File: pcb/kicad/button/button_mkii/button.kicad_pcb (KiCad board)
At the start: 2 copper layers, 168 parts, among them J1 SWD with less, U1 STBlueNRG-1, Y1 Xtal 32.768kHz, Y2 XTAL 16MHz

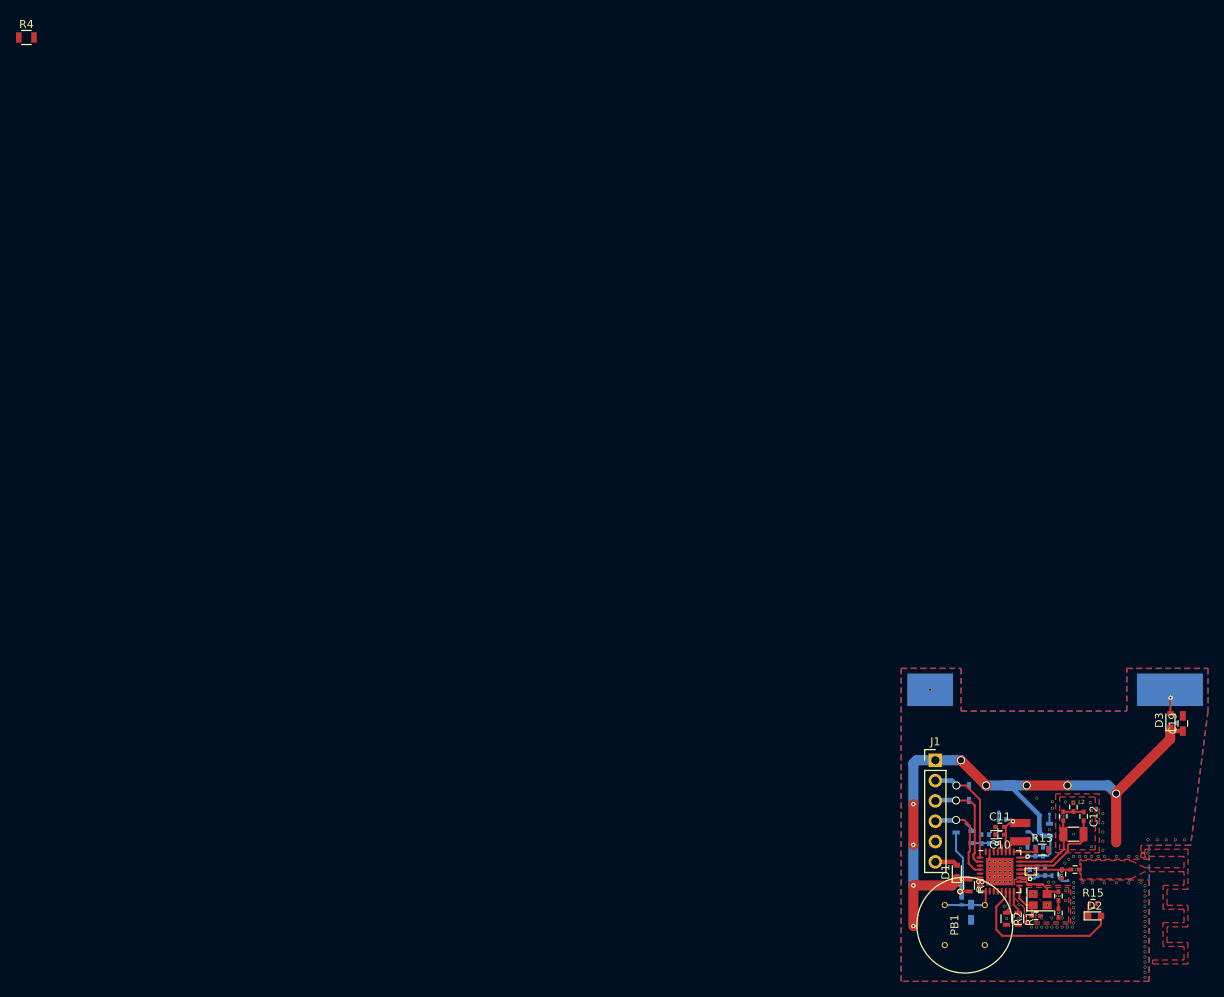
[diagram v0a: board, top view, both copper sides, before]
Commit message: updated design, layout, and appnotes; rev3
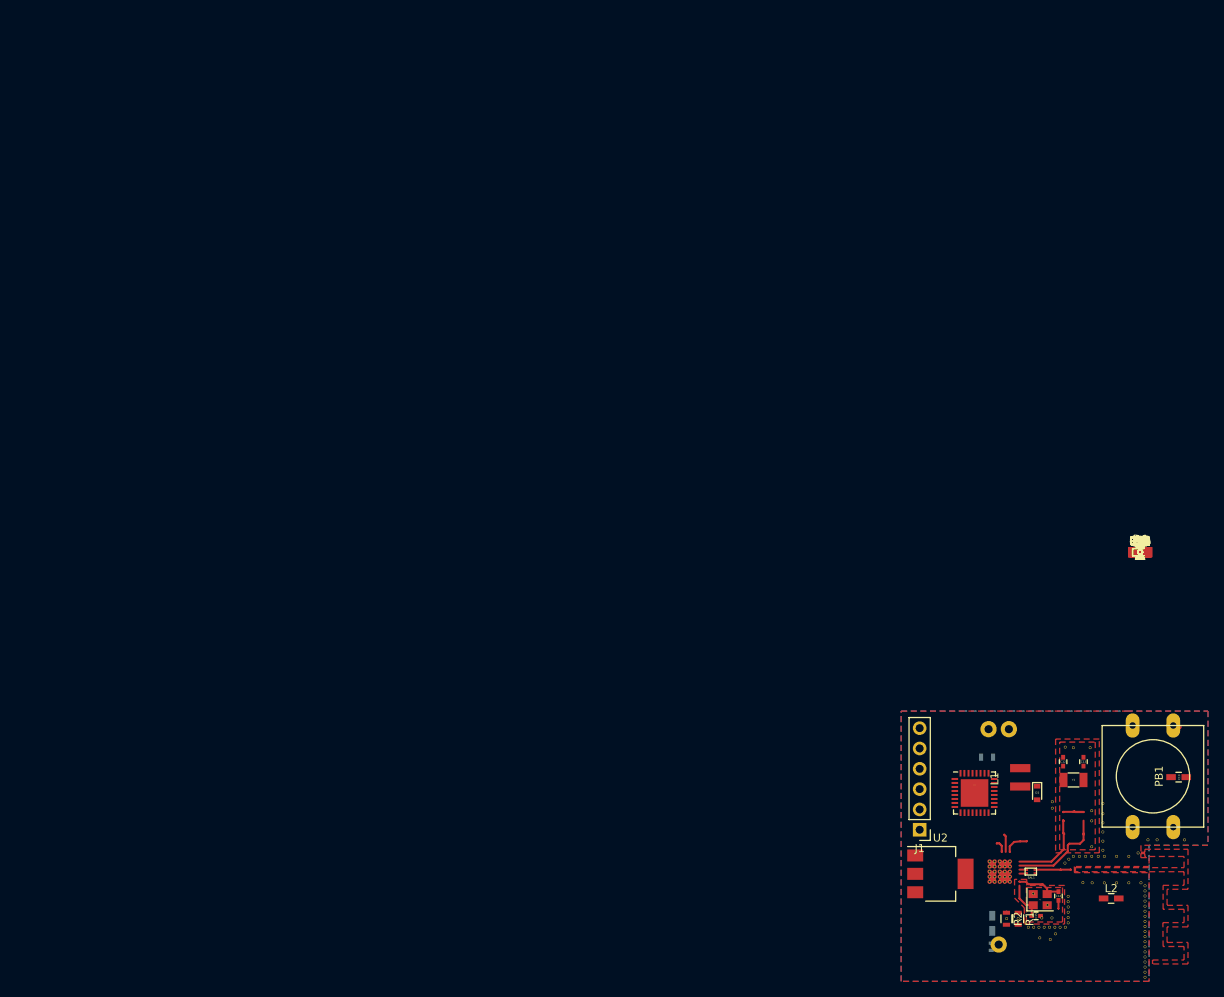
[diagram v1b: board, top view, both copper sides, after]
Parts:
- removed L3: RFC, Miscellaneous:L_0402
- removed the REF** at (127.9, 99.0)
- removed the REF** at (122.2, 108.6)
- removed the REF** at (130.9, 105.6)
- removed the REF** at (124.2, 101.3)
- removed the REF** at (130.9, 106.2)
- removed the REF** at (124.1, 108.4)
- removed the REF** at (113.0, 81.5)
- removed the REF** at (140.2, 101.9)
- removed the REF** at (130.9, 106.9)
- removed the REF** at (143.6, 100.3)
- removed the REF** at (142.5, 100.3)
- removed the REF** at (127.8, 105.6)
- removed the REF** at (128.4, 105.6)
- removed the REF** at (130.9, 107.5)
- added C20, C21: 1uF, Capacitors_SMD:C_0402, F.Cu at (139.2, 64.3)
- added C22: 1uF, Capacitors_SMD:C_0805, F.Cu at (139.2, 64.3)
- added C23: 0.1uF, Capacitors_SMD:C_0603, F.Cu at (139.2, 64.3)
- added C24: 0.01uF, Capacitors_SMD:C_0402, F.Cu at (139.2, 64.3)
- added R16: 1k, Resistors_SMD:R_0402, F.Cu at (139.2, 64.3)
- added R17: 100k, Resistors_SMD:R_0402, F.Cu at (139.2, 64.3)
- added TP7: Xtal32MHz, Miscellaneous:Measurement_Point_Round-SMD-tiniest, F.Cu at (139.2, 64.3)
- added TP8: Xtal32kHz, Miscellaneous:Measurement_Point_Round-SMD-tiniest, F.Cu at (139.2, 64.3)
- added U2: TLV1117LV-3V, TO_SOT_Packages_SMD:SOT-223, F.Cu at (114.2, 104.5)
- BT1: footprint Batteries:SMD_CoinCell -> Batteries:CoinCell_holder_1060x630
- C1: value 100pF -> 1uF; footprint Capacitors_SMD:C_0402 -> Capacitors_SMD:C_0805; moved to F.Cu
- C14: value 22pF -> 27pF
- C15: value 18pF -> 33pF
- C18: value CP -> 1uF
- C2: footprint Capacitors_SMD:C_0402 -> Capacitors_SMD:C_0603; moved to F.Cu
- C3: value 2.2pF -> 0.01uF; moved to F.Cu
- C4: value 1000pF -> 0.01uF; footprint Capacitors_SMD:C_0402 -> Capacitors_SMD:C_0805; moved to F.Cu
- C5: value 2.2uF -> 1000pF; footprint Capacitors_SMD:C_0402 -> Capacitors_SMD:C_0603; moved to F.Cu
- C6, R10, R11, R12, R3, R7, R9, TP1, TP3, TP4, TP5, TP6: moved to F.Cu
- C7: value 10pF -> 0.01uF; footprint Capacitors_SMD:C_0402 -> Capacitors_SMD:C_0805; moved to F.Cu
- C8: value 1uF -> 1000pF; footprint Capacitors_SMD:C_0402 -> Capacitors_SMD:C_0603; moved to F.Cu
- C9: value 1000pF -> 10pF; moved to F.Cu
- D1: value Power thru SWD -> LED (Green-1); footprint Diodes_SMD:D_0603 -> LEDs:LED_0402
- D2: value LED -> LED (Green-2); footprint LEDs:LED_0603 -> LEDs:LED_0402
- L2: value RFC -> L; footprint Miscellaneous:L_0402 -> Capacitors_SMD:C_0603_HandSoldering
- PB1: value pb_basic -> pb_v2; footprint Miscellaneous:pb_basic -> Buttons_Switches_THT:SW_PUSH-12mm
- R14: value 10k -> 1k
- R6: value 100k -> 1k; footprint Resistors_SMD:R_0603 -> Resistors_SMD:R_0402; moved to F.Cu
- U1: footprint uCs:STBNRG1 -> STBNRG1
- Y2: value XTAL 16MHz -> XTAL 32MHz
- moved R4 153.4 mm to (139.2, 64.3)
- moved TP2 48.0 mm to (139.2, 64.3)
- moved R8 46.8 mm to (139.2, 64.3), turned to 0 degrees
- moved D1 46.1 mm to (139.2, 64.3), turned to 0 degrees
- moved D2 45.8 mm to (139.2, 64.3)
- moved R15 44.3 mm to (139.2, 64.3)
- moved C5 42.5 mm to (139.2, 64.3), turned to 0 degrees
- moved TP3 42.0 mm to (139.2, 64.3)
- moved C6 41.9 mm to (139.2, 64.3), turned to 0 degrees
- moved R9 41.8 mm to (139.2, 64.3)
- moved C4 41.6 mm to (139.2, 64.3), turned to 0 degrees
- moved C16 41.4 mm to (139.2, 64.3), turned to 0 degrees
- moved R7 41.3 mm to (139.2, 64.3), turned to 0 degrees
- moved R6 41.3 mm to (139.2, 64.3), turned to 0 degrees
- moved C3 41.0 mm to (139.2, 64.3), turned to 0 degrees
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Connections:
- net RF0 renamed /RF0
- net RF1 renamed /RF1
- BT1 pad 2: GND -> Net-(BT1-Pad1)
- C12 pad 1: Net-(C12-Pad1) -> GND
- C13 pad 1: Net-(C12-Pad1) -> GND
- C14 pad 1: Net-(C14-Pad1) -> GND
- C17 pad 2: Net-(BAL1-Pad3) -> GND
- C18 pad 1: DIO3 -> +3V3
- C18 pad 2: GND -> /DIO12_BUTTON
- C19 pad 1: +3V3 -> Net-(BT1-Pad1)
- C4 pad 1: GND -> +3V3
- C4 pad 2: +3V3 -> GND
- C5 pad 1: GND -> +3V3
- C5 pad 2: +3V3 -> GND
- C6 pad 1: GND -> +3V3
- C6 pad 2: +3V3 -> GND
- D1 pad 1: +3V3 -> GND
- D2 pad 2: ANATEST1 -> /DIO3_LED
- J1 pad 1: +3V3 -> Net-(C20-Pad2)
- J1 pad 2: DIO10 -> DIO7
- J1 pad 4: DIO7 -> DIO10
- J1 pad 6: Net-(D1-Pad2) -> +3V3
- L2 pad 1: Net-(C12-Pad1) -> Net-(BAL1-Pad3)
- PB1 pad 1: DIO3 -> +3V3
- PB1 pad 2: GND -> /DIO12_BUTTON
- R13 pad 1: RESET -> GND
- R13 pad 2: GND -> Net-(R13-Pad2)
- R14 pad 1: +3V3 -> /DIO12_BUTTON
- R14 pad 2: DIO3 -> Net-(D1-Pad2)
- R4 pad 1: DIO10 -> +3V3
- R4 pad 2: +3V3 -> DIO7
- R6 pad 1: DIO7 -> Net-(C14-Pad2)
- R6 pad 2: +3V3 -> Net-(R6-Pad2)
- R7 pad 1: Net-(C1-Pad1) -> Net-(R7-Pad1)
- R7 pad 2: Net-(R7-Pad2) -> Net-(C1-Pad1)
- R8 pad 1: +3V3 -> Net-(R8-Pad1)
- R8 pad 2: Net-(R8-Pad2) -> +3V3
- TP1 pad 1: Net-(R7-Pad2) -> Net-(R7-Pad1)
- TP2 pad 1: Net-(R8-Pad2) -> Net-(R8-Pad1)
- U1 pad 14: ANATEST1 -> Net-(U1-Pad14)
- U1 pad 25: RESET -> Net-(R13-Pad2)
- U1 pad 30: Net-(U1-Pad30) -> /DIO12_BUTTON
- U1 pad 9: DIO3 -> /DIO3_LED
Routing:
- net +3V3: track 104.9 -> 1.14 mm, vias 12 -> 0
- net (no net): track 0.00 -> 34.6 mm
- net ANATEST1: track 20.4 -> 0.00 mm
- net DIO10: track 14.2 -> 0.00 mm, vias 1 -> 0
- net Net-(C13-Pad2): track 14.2 -> 0.00 mm
- net DIO9: track 13.3 -> 0.00 mm, vias 1 -> 0
- net DIO7: track 11.4 -> 0.00 mm, vias 1 -> 0
- net Net-(C12-Pad2): track 8.43 -> 0.00 mm
- net Net-(C10-Pad1): track 7.19 -> 0.00 mm, vias 1 -> 0
- net DIO3: track 6.94 -> 0.00 mm
- net Net-(C1-Pad1): track 4.65 -> 0.00 mm, vias 1 -> 0
- net Net-(BT1-Pad1): track 4.63 -> 0.00 mm, vias 1 -> 0
- net RESET: track 3.17 -> 0.00 mm
- net ADC2: track 2.91 -> 0.01 mm
- net Net-(D1-Pad2): track 2.87 -> 0.00 mm
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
